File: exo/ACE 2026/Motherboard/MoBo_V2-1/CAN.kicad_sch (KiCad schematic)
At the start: 7 parts, among them U501 MAX3221

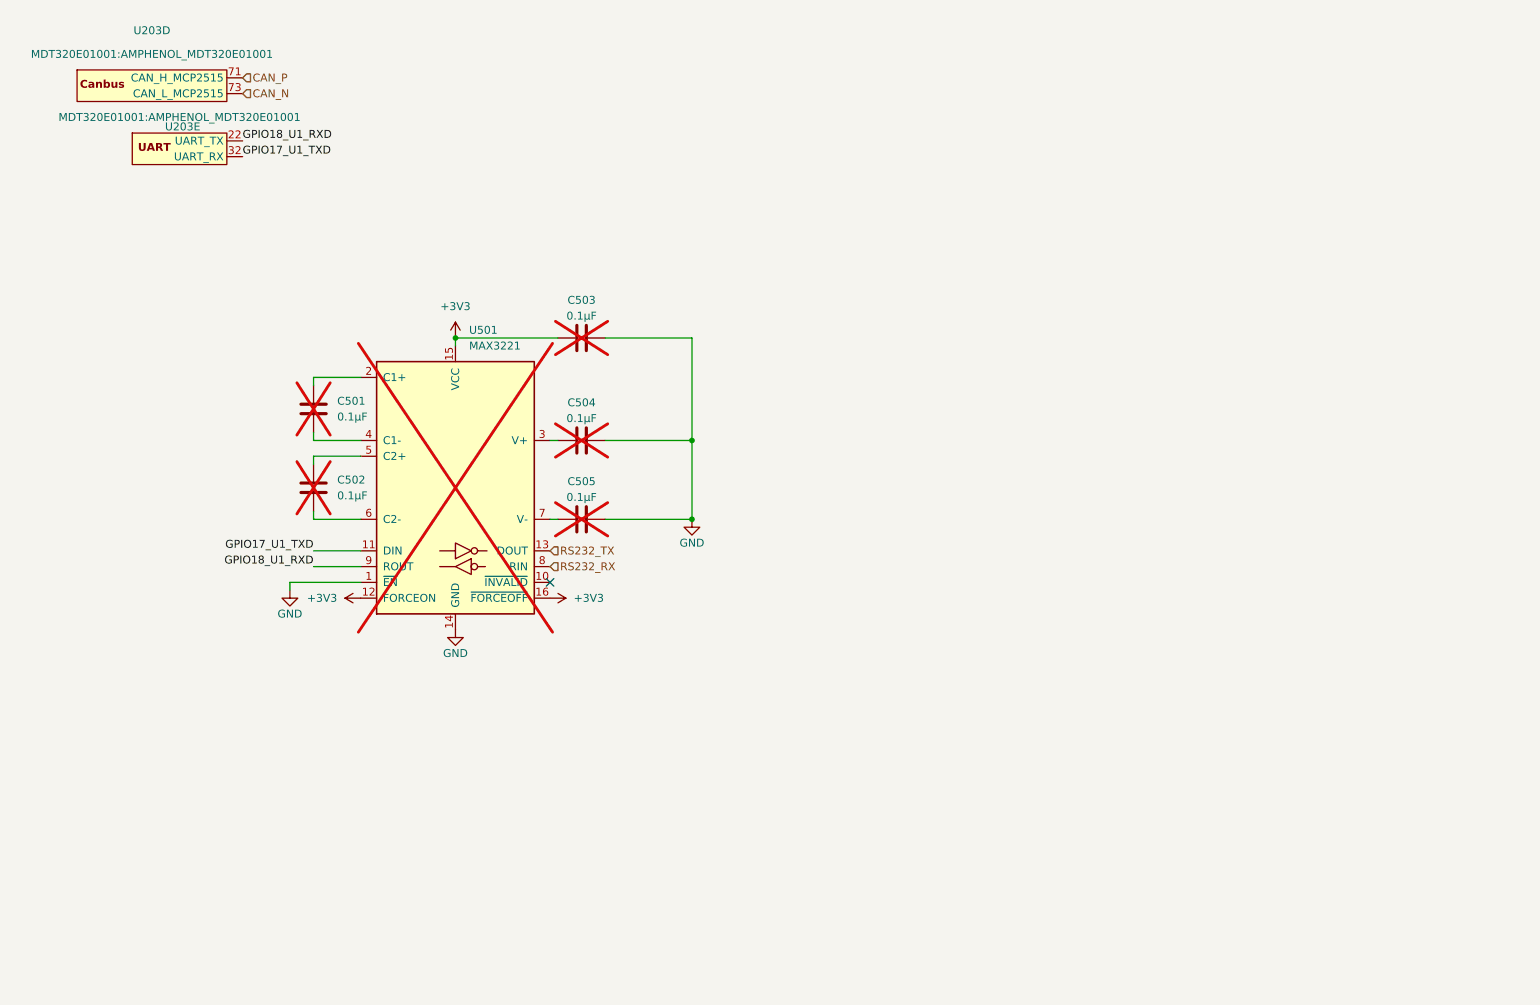
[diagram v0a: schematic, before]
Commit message: Pushing changed files
multiple correctiosn done especially a new Mobo
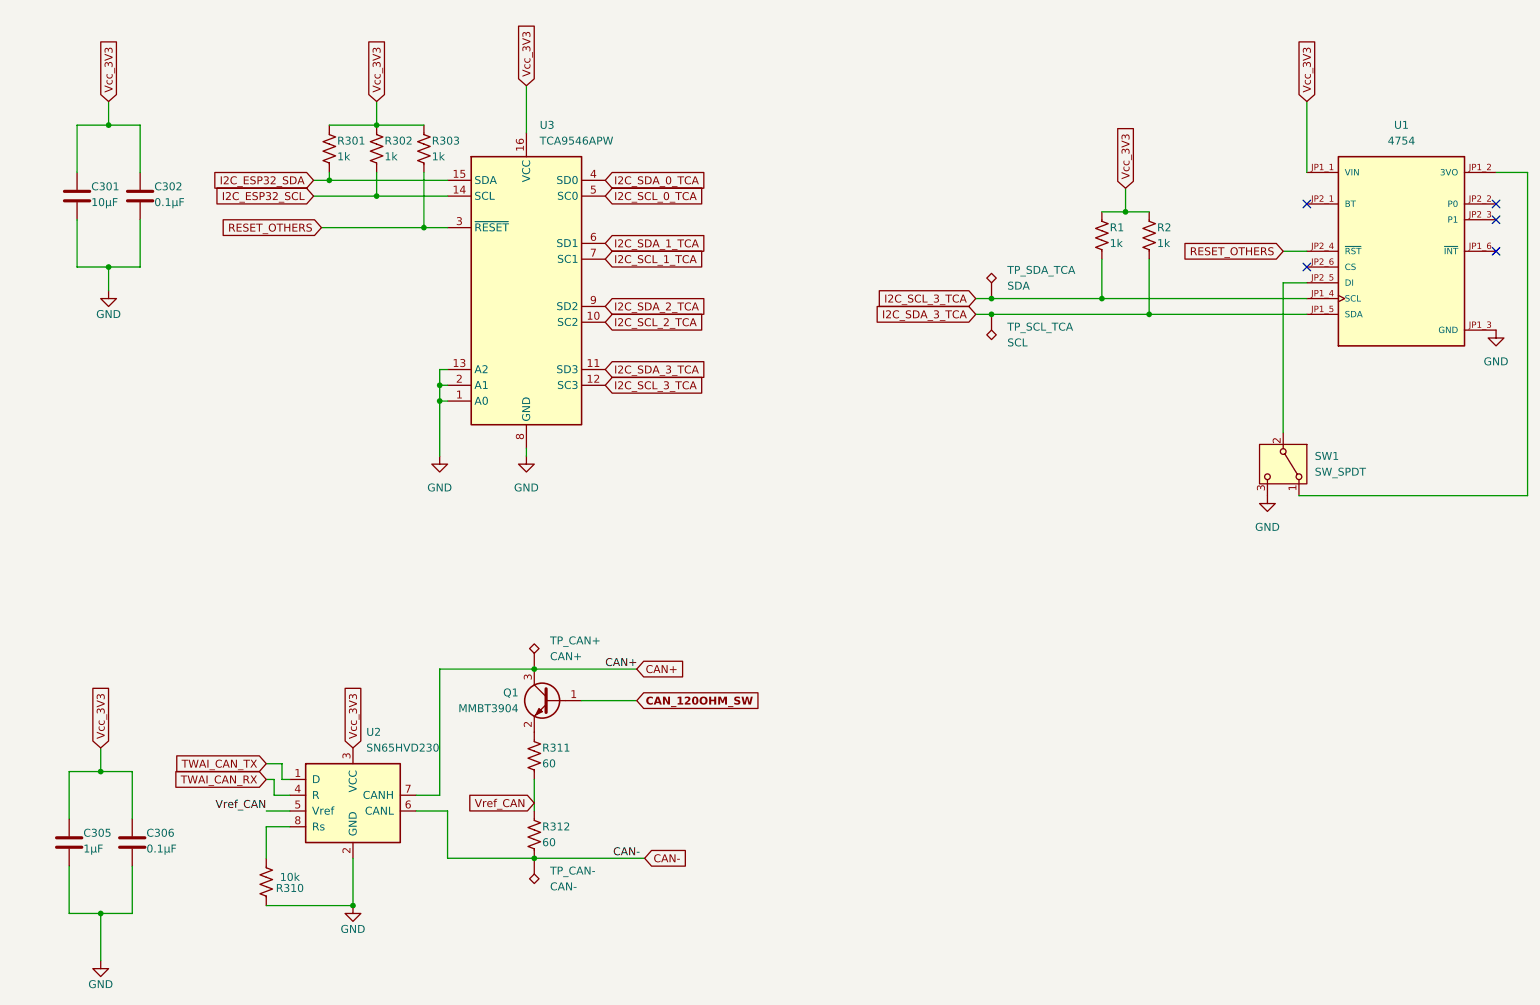
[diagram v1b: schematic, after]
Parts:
- removed C501, C502, C503, C504, C505: 0.1µF, Capacitor_SMD:C_0603_1608Metric_Pad1.08x0.95mm_HandSolder, symbol Device:C
- removed U203: ~, MDT320E01001:AMPHENOL_MDT320E01001, symbol connecteur_m2_key_E:connecteur_SOM_ESP32_V2
- removed U501: MAX3221, Package_SO:SSOP-16_3.9x4.9mm_P0.635mm, symbol Interface_UART:MAX3221
- added C301: 10µF, Resistor_SMD:R_0805_2012Metric, symbol Device:C
- added C302, C306: 0.1µF, Resistor_SMD:R_0805_2012Metric, symbol Device:C
- added C305: 1µF, Resistor_SMD:R_0805_2012Metric, symbol Device:C
- added Q1: MMBT3904, Package_TO_SOT_SMD:SOT-23-3, symbol Transistor_BJT:MMBT3904
- added R1, R2, R301, R302, R303: 1k, Resistor_SMD:R_0805_2012Metric, symbol Device:R_US
- added R310: 10k, Resistor_SMD:R_0805_2012Metric, symbol Device:R_US
- added R311, R312: 60, Resistor_SMD:R_0805_2012Metric, symbol Device:R_US
- added SW1: SW_SPDT, Button_Switch_SMD:SW_SPDT_CK_JS102011SAQN, symbol Switch:SW_SPDT
- added TP_CAN+: CAN+, Connector_PinHeader_2.54mm:PinHeader_1x01_P2.54mm_Vertical, symbol Connector:TestPoint_Alt
- added TP_CAN-: CAN-, Connector_PinHeader_2.54mm:PinHeader_1x01_P2.54mm_Vertical, symbol Connector:TestPoint_Alt
- added TP_SCL_TCA: SCL, Connector_PinHeader_2.54mm:PinHeader_1x01_P2.54mm_Vertical, symbol Connector:TestPoint_Alt
- added TP_SDA_TCA: SDA, Connector_PinHeader_2.54mm:PinHeader_1x01_P2.54mm_Vertical, symbol Connector:TestPoint_Alt
- added U1: 4754, Biogenius:MODULE_4754, symbol 4754:4754
- added U2: SN65HVD230, Package_SO:SOIC-8_3.9x4.9mm_P1.27mm, symbol Interface_CAN_LIN:SN65HVD230
- added U3: TCA9546APW, Package_SO:TSSOP-16_4.4x5mm_P0.65mm, symbol Interface_Expansion:TCA9546APW
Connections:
- net GND: now also C301.2, C302.2, C305.2, C306.2, R310.1, SW1.3 (C), U1.JP1_3 (GND), U2.2 (GND), U3.1 (A0), U3.13 (A2), U3.2 (A1), U3.8 (GND)
- new net: SW1.1 (A), U1.JP1_2 (3VO)
- new net: SW1.2 (B), U1.JP2_5 (DI)
- new net: R310.2, U2.8 (Rs)
- new net: Q1.2 (E), R311.1
- new net CAN+: Q1.3 (C), TP_CAN+.1, U2.7 (CANH)
- new net CAN-: R312.2, TP_CAN-.1, U2.6 (CANL)
- new net CAN_120OHM_SW: Q1.1 (B)
- new net I2C_ESP32_SCL: R302.2, U3.14 (SCL)
- new net I2C_ESP32_SDA: R301.2, U3.15 (SDA)
- new net I2C_SCL_0_TCA: U3.5 (SC0)
- new net I2C_SCL_1_TCA: U3.7 (SC1)
- new net I2C_SCL_2_TCA: U3.10 (SC2)
- new net I2C_SCL_3_TCA: R1.2, TP_SDA_TCA.1, U1.JP1_4 (SCL), U3.12 (SC3)
- new net I2C_SDA_0_TCA: U3.4 (SD0)
- new net I2C_SDA_1_TCA: U3.6 (SD1)
- new net I2C_SDA_2_TCA: U3.9 (SD2)
- new net I2C_SDA_3_TCA: R2.2, TP_SCL_TCA.1, U1.JP1_5 (SDA), U3.11 (SD3)
- new net RESET_OTHERS: R303.2, U1.JP2_4 (~{RST}), U3.3 (~{RESET})
- new net TWAI_CAN_RX: U2.4 (R)
- new net TWAI_CAN_TX: U2.1 (D)
- new net Vcc_3V3: C301.1, C302.1, C305.1, C306.1, R1.1, R2.1, R301.1, R302.1, R303.1, U1.JP1_1 (VIN), U2.3 (VCC), U3.16 (VCC)
- new net Vref_CAN: R311.2, R312.1, U2.5 (Vref)
- no-connect marks 1 -> 5
